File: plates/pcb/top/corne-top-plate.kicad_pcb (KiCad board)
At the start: 2 copper layers, 132.9 x 91.4 mm, 26 parts, among them SW2 KEY_SWITCH

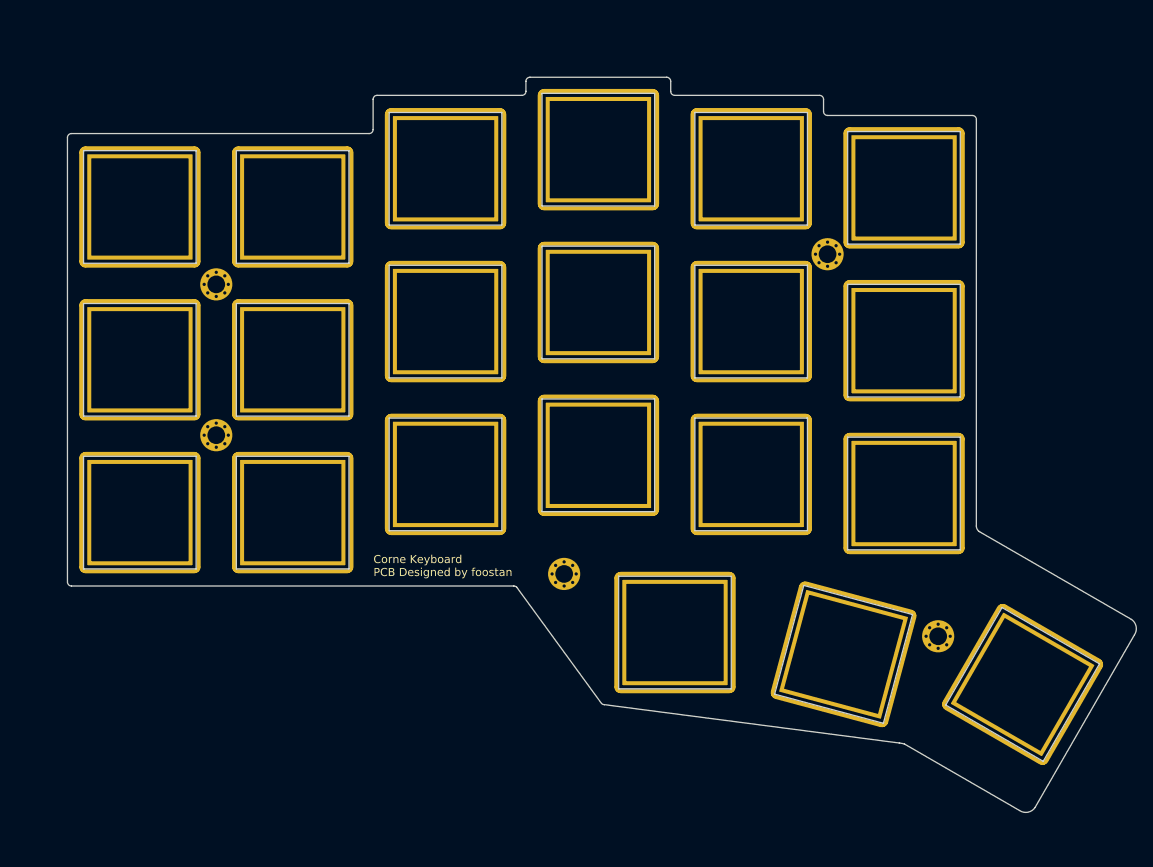
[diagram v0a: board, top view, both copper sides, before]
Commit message: rp2040 v0
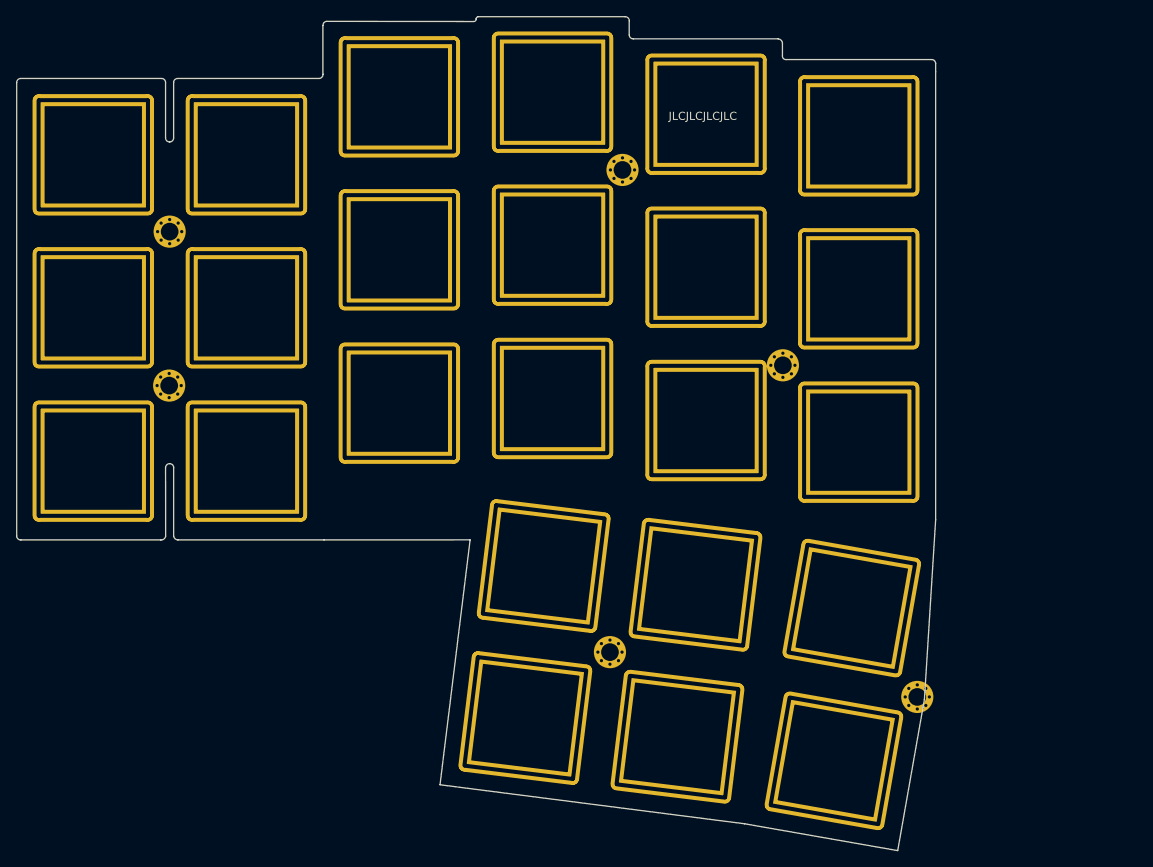
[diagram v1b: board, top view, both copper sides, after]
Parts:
- removed the ? at (122.8, 122.8)
- removed the ? at (169.2, 130.5)
- removed the ? at (79.5, 105.5)
- removed the ? at (155.5, 83.0)
- removed the ? at (79.5, 86.8)
- removed the SW2 at (179.8, 136.5)
- removed the SW2 at (127.0, 89.0)
- removed the SW2 at (127.0, 108.0)
- removed the SW2 at (127.0, 70.0)
- removed the SW2 at (108.0, 91.4)
- removed the SW2 at (108.0, 110.4)
- removed the SW2 at (108.0, 72.4)
- removed the SW2 at (89.0, 96.1)
- removed the SW2 at (89.0, 115.1)
- removed the SW2 at (70.0, 115.1)
- removed the SW2 at (157.5, 132.7)
- removed the SW2 at (70.0, 96.1)
- removed the SW2 at (70.0, 77.1)
- removed the SW2 at (136.5, 130.0)
- removed the SW2 at (165.0, 112.8)
- removed the SW2 at (165.0, 74.8)
- removed the SW2 at (165.0, 93.8)
- removed the SW2 at (146.0, 91.4)
- removed the SW2 at (146.0, 72.4)
- removed the SW2 at (146.0, 110.4)
- added ?: , kbd:M2_HOLE_v3, F.Cu at (166.7, 138.0)
- added ?: , kbd:M2_HOLE_v3, F.Cu at (128.4, 132.5)
- added ?: , kbd:M2_HOLE_v3, F.Cu at (149.9, 96.8)
- added ?: , kbd:M2_HOLE_v3, F.Cu at (130.0, 72.5)
- added ?: , kbd:M2_HOLE_v3, F.Cu at (73.6, 99.3)
- added ?: , kbd:M2_HOLE_v3, F.Cu at (73.7, 80.2)
- added SW2: KEY_SWITCH, kbd:SW_Hole_TH, F.Cu at (102.3, 63.4)
- added SW2: KEY_SWITCH, kbd:SW_Hole_TH, F.Cu at (121.3, 100.9)
- added SW2: KEY_SWITCH, kbd:SW_Hole_TH, F.Cu at (83.2, 70.6)
- added SW2: KEY_SWITCH, kbd:SW_Hole_TH, F.Cu at (140.4, 84.6)
- added SW2: KEY_SWITCH, kbd:SW_Hole_TH, F.Cu at (121.3, 81.9)
- added SW2: KEY_SWITCH, kbd:SW_Hole_TH, F.Cu at (83.2, 108.7)
- added SW2: KEY_SWITCH, kbd:SW_Hole_TH, F.Cu at (159.4, 87.3)
- added SW2: KEY_SWITCH, kbd:SW_Hole_TH, F.Cu at (156.3, 146.0)
- added SW2: KEY_SWITCH, kbd:SW_Hole_TH, F.Cu at (64.2, 108.7)
- added SW2: KEY_SWITCH, kbd:SW_Hole_TH, F.Cu at (139.1, 124.1)
- added SW2: KEY_SWITCH, kbd:SW_Hole_TH, F.Cu at (121.3, 62.9)
- added SW2: KEY_SWITCH, kbd:SW_Hole_TH, F.Cu at (120.2, 121.8)
- added SW2: KEY_SWITCH, kbd:SW_Hole_TH, F.Cu at (102.3, 82.5)
- added SW2: KEY_SWITCH, kbd:SW_Hole_TH, F.Cu at (136.8, 143.0)
- added SW2: KEY_SWITCH, kbd:SW_Hole_TH, F.Cu at (158.5, 127.0)
- added SW2: KEY_SWITCH, kbd:SW_Hole_TH, F.Cu at (140.4, 103.7)
- added SW2: KEY_SWITCH, kbd:SW_Hole_TH, F.Cu at (117.9, 140.7)
- added SW2: KEY_SWITCH, kbd:SW_Hole_TH, F.Cu at (140.4, 65.6)
- added SW2: KEY_SWITCH, kbd:SW_Hole_TH, F.Cu at (83.2, 89.7)
- added SW2: KEY_SWITCH, kbd:SW_Hole_TH, F.Cu at (102.3, 101.5)
- added SW2: KEY_SWITCH, kbd:SW_Hole_TH, F.Cu at (64.2, 89.7)
- added SW2: KEY_SWITCH, kbd:SW_Hole_TH, F.Cu at (159.4, 68.3)
- added SW2: KEY_SWITCH, kbd:SW_Hole_TH, F.Cu at (159.4, 106.4)
- moved SW2 25.6 mm to (64.2, 70.6)
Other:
- board size 132.9 x 91.4 mm -> 114.3 x 103.7 mm
- net class Default removed
- board text added: "JLCJLCJLCJLC"
- board text removed: "Corne Keyboard PCB Designed by foostan"
